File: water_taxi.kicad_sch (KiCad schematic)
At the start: 18 parts

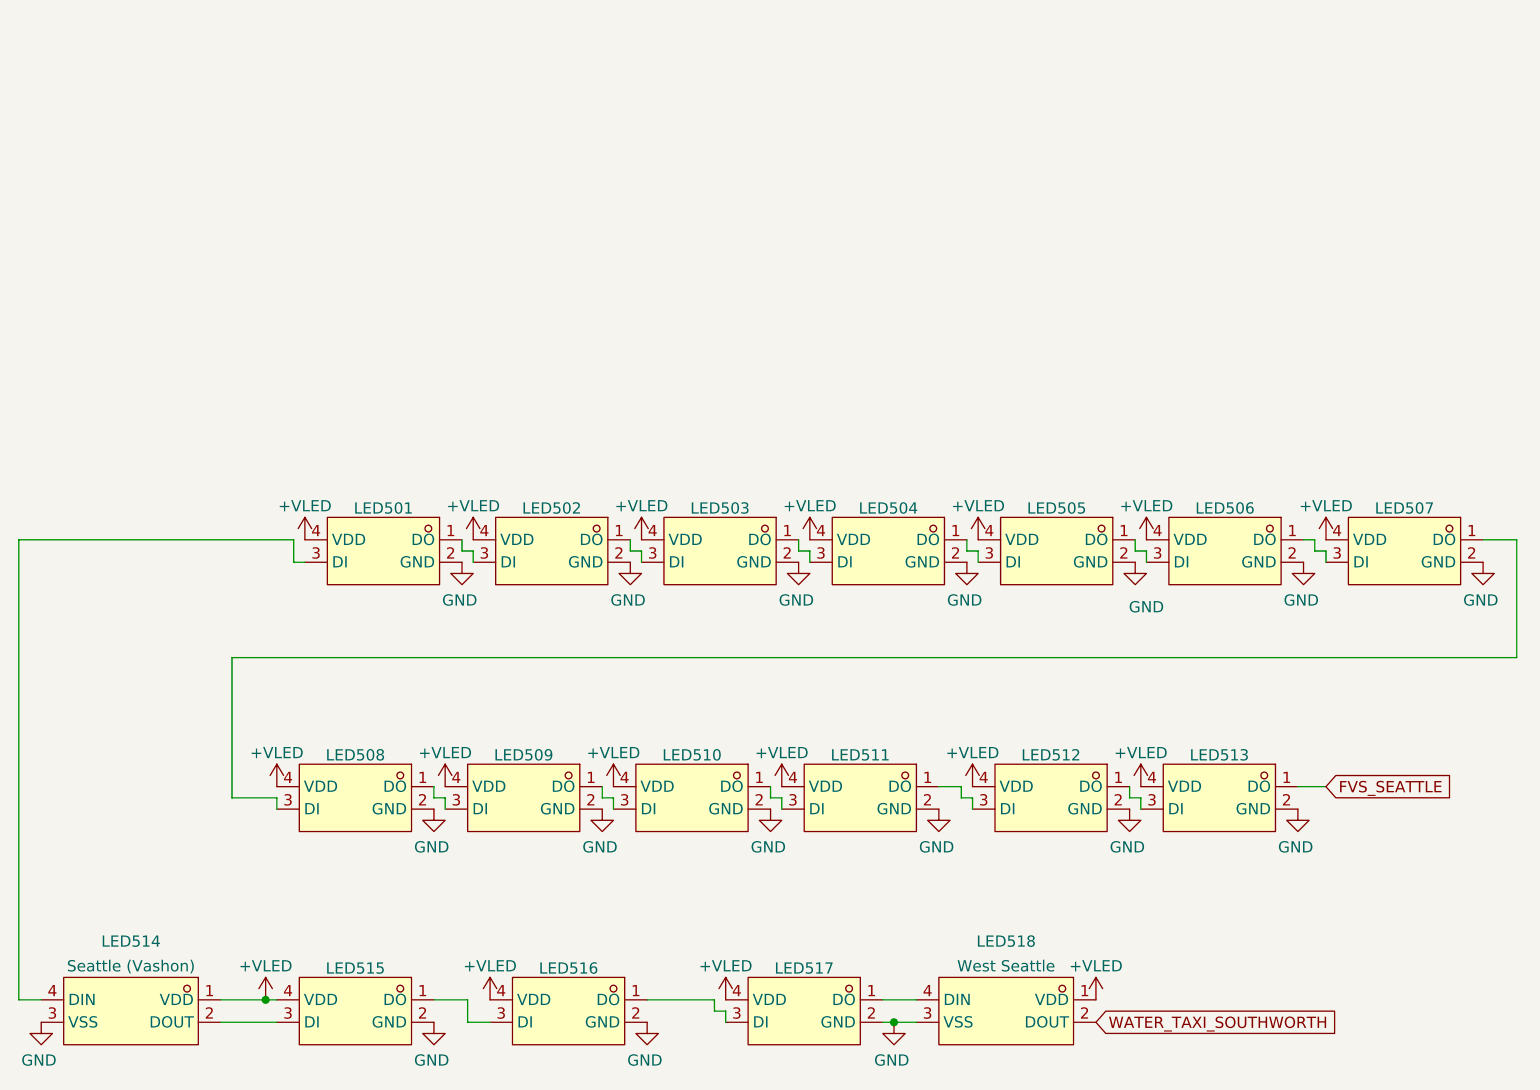
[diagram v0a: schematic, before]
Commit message: rev-b validation run
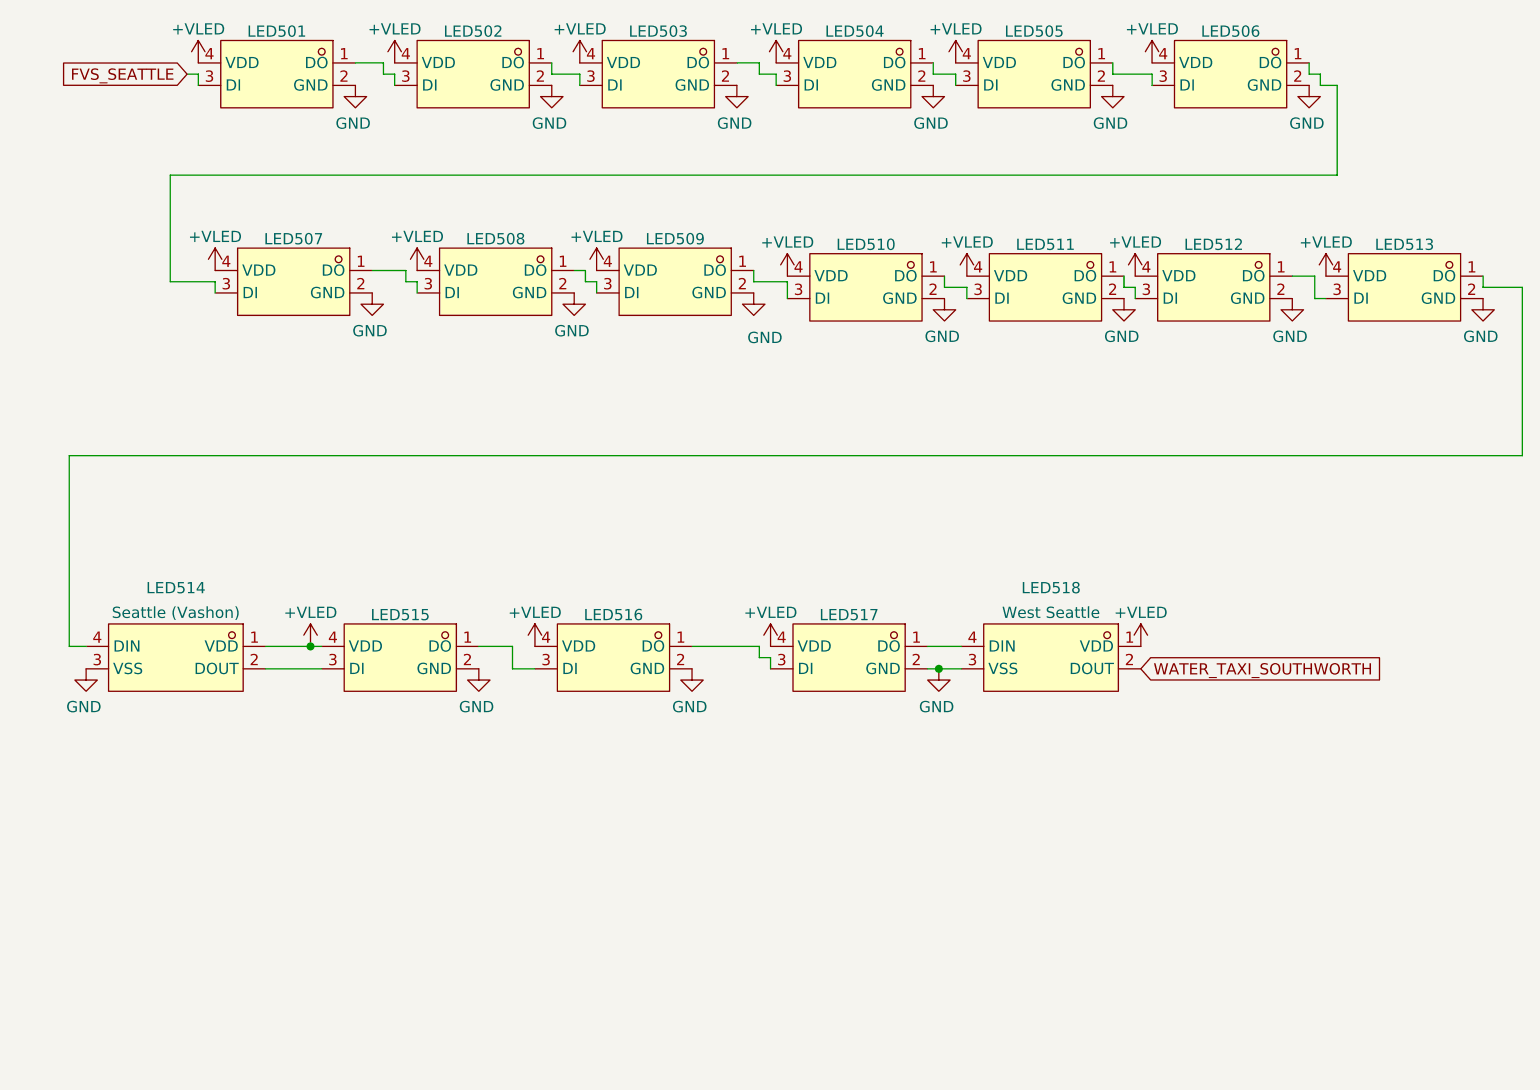
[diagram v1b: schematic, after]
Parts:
- LED501, LED502, LED503, LED504, LED505, LED506, LED507, LED508, LED509, LED510, LED511, LED512, LED513, LED515, LED516, LED517: LCSC Part C965555 -> C52917434
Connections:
- net FVS_SEATTLE: now also LED501.3 (DI); no longer LED513.1 (DO)
- net at LED514.4 (DIN): now also LED513.1 (DO); no longer LED501.3 (DI)
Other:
- moved on the sheet: LED514, LED515, LED516, LED517, LED518
